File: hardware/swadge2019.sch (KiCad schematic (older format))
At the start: 18 parts, among them SW1 TACTILE, SW2 TACTILE, SW3 TACTILE, SW4 TACTILE, SW5 TACTILE, SW6 TACTILE

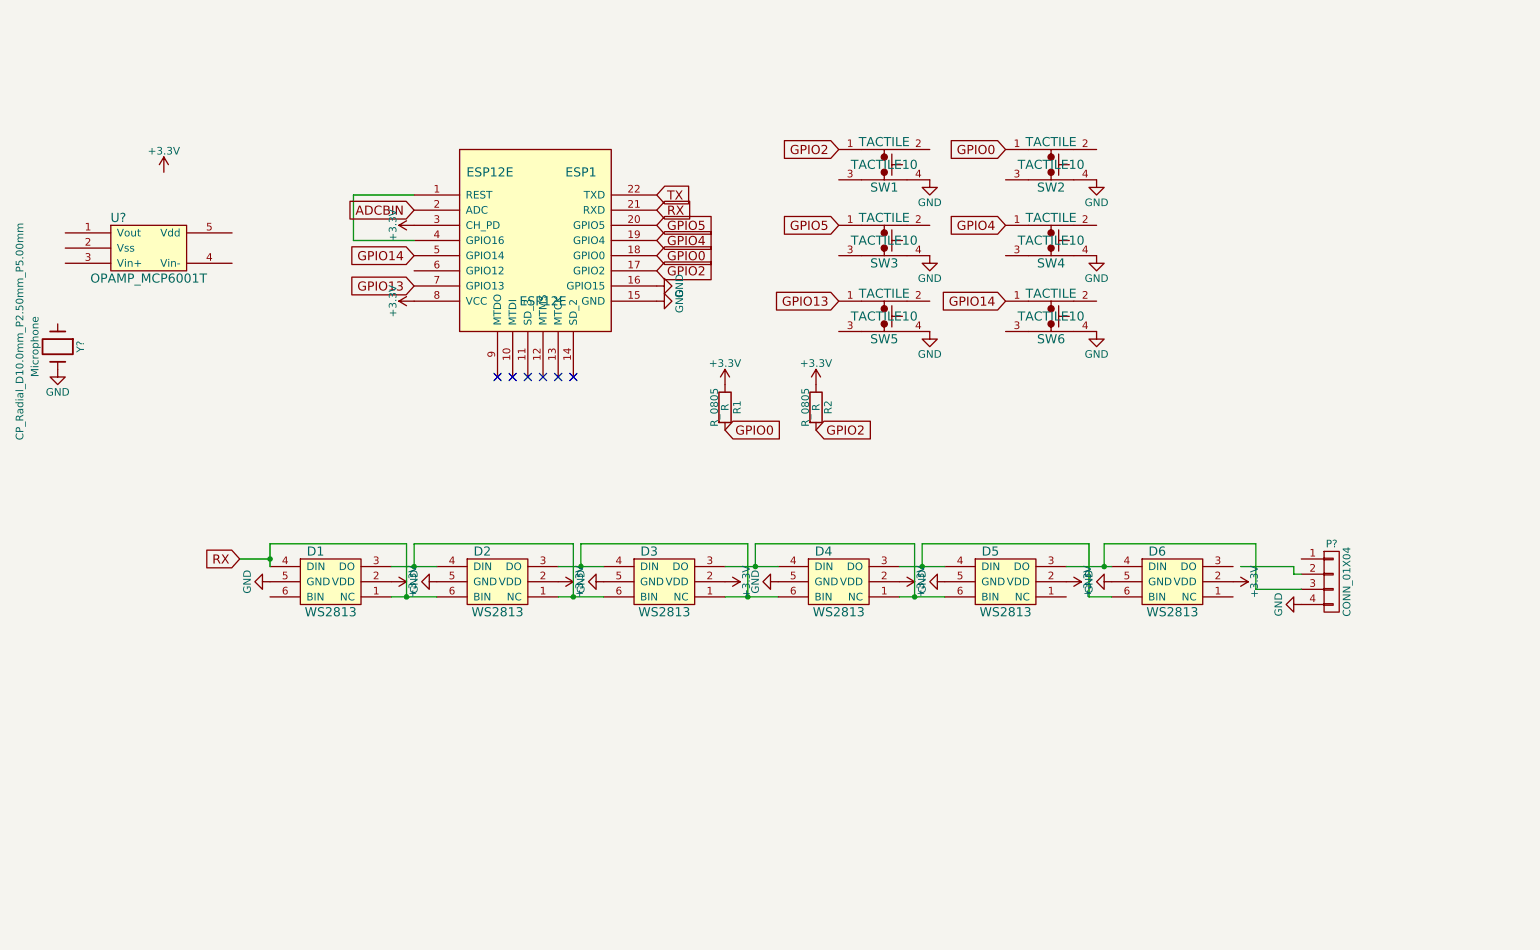
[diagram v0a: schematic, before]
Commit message: bump design
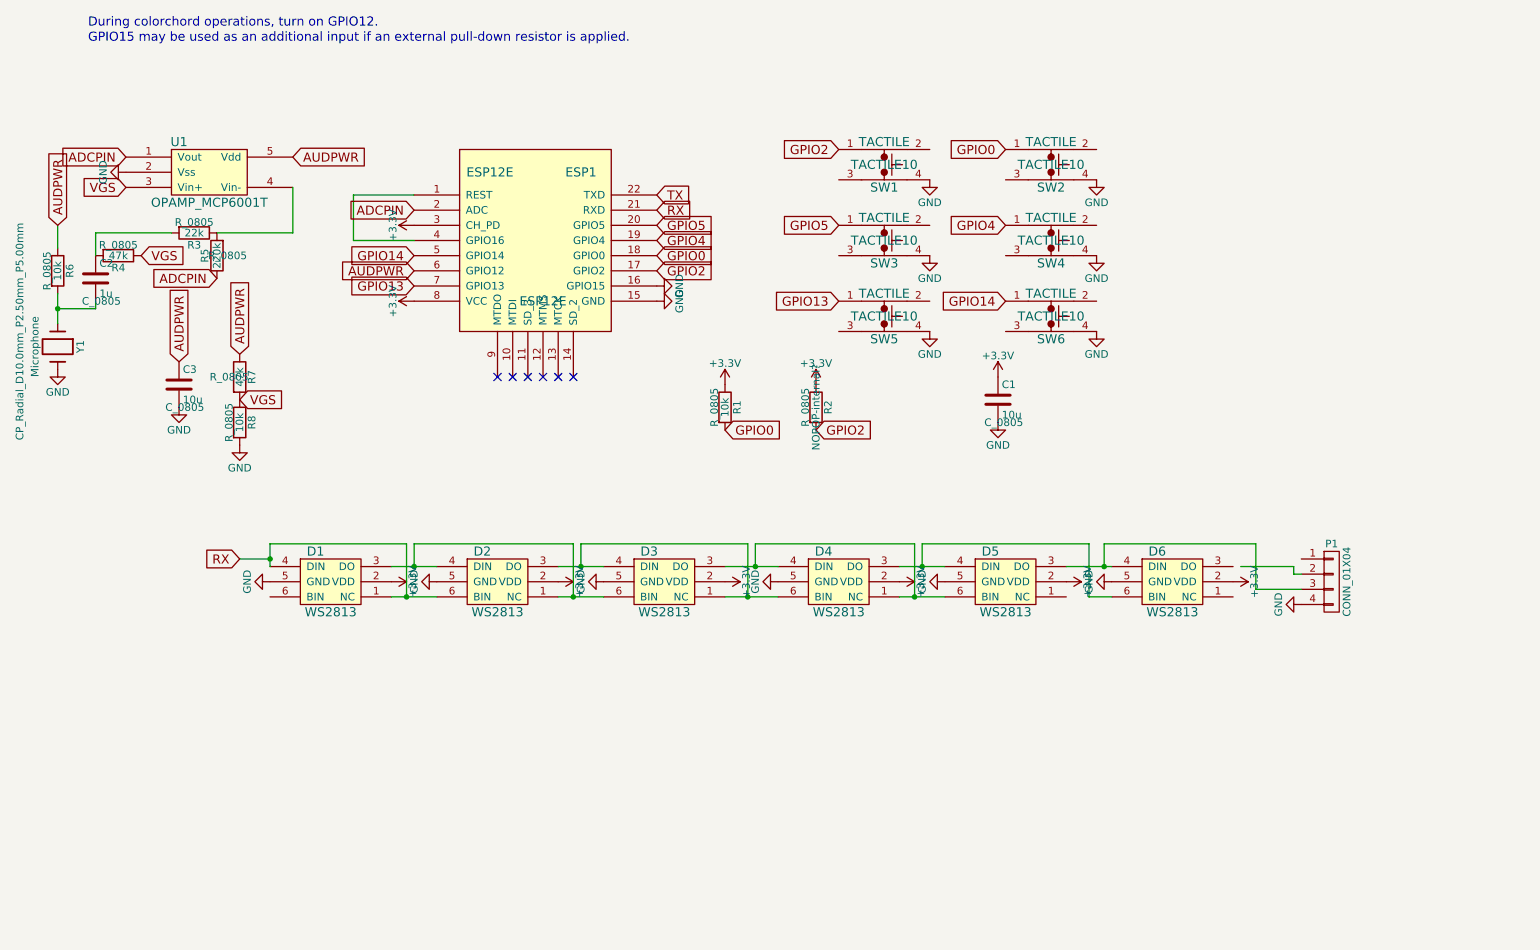
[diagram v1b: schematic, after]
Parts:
- added C1, C3: 10u, C_0805, symbol C
- added C2: 1u, C_0805, symbol C
- added R3: 22k, R_0805, symbol R
- added R4, R7: 47k, R_0805, symbol R
- added R5: 220k, R_0805, symbol R
- added R6, R8: 10k, R_0805, symbol R
- R1: value R -> 10k
- R2: value R -> NOPOP-internal?
- gave numbers to parts that had none: 3
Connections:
- net ADCBIN is gone; now on net ADCPIN: ESP1.2 (ADC)
- net +3V3: now also C1.1
- net GND: now also U1.2 (Vss), C1.2, C3.2, R8.2
- net AUDPWR: now reaches ESP1.6 (GPIO12)
- net AUDPWR: now also U1.5 (Vdd), C3.1, R6.1, R7.1
- net ADCPIN: now reaches U1.1 (Vout)
- net ADCPIN: now also R5.1
- net VGS: now reaches U1.3 (Vin+)
- net VGS: now also R4.1, R7.2, R8.1
- net at U1.4 (Vin-): now also R3.1, R5.2
- net at Y1.1: now also C2.2, R6.2
- new net: C2.1, R3.2, R4.2
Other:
- note added: "During colorchord operations, turn on GPIO12."
- note added: "GPIO15 may be used as an additional input if an external pull-down resistor is applied."
- moved on the sheet: U1

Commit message: update swadge set
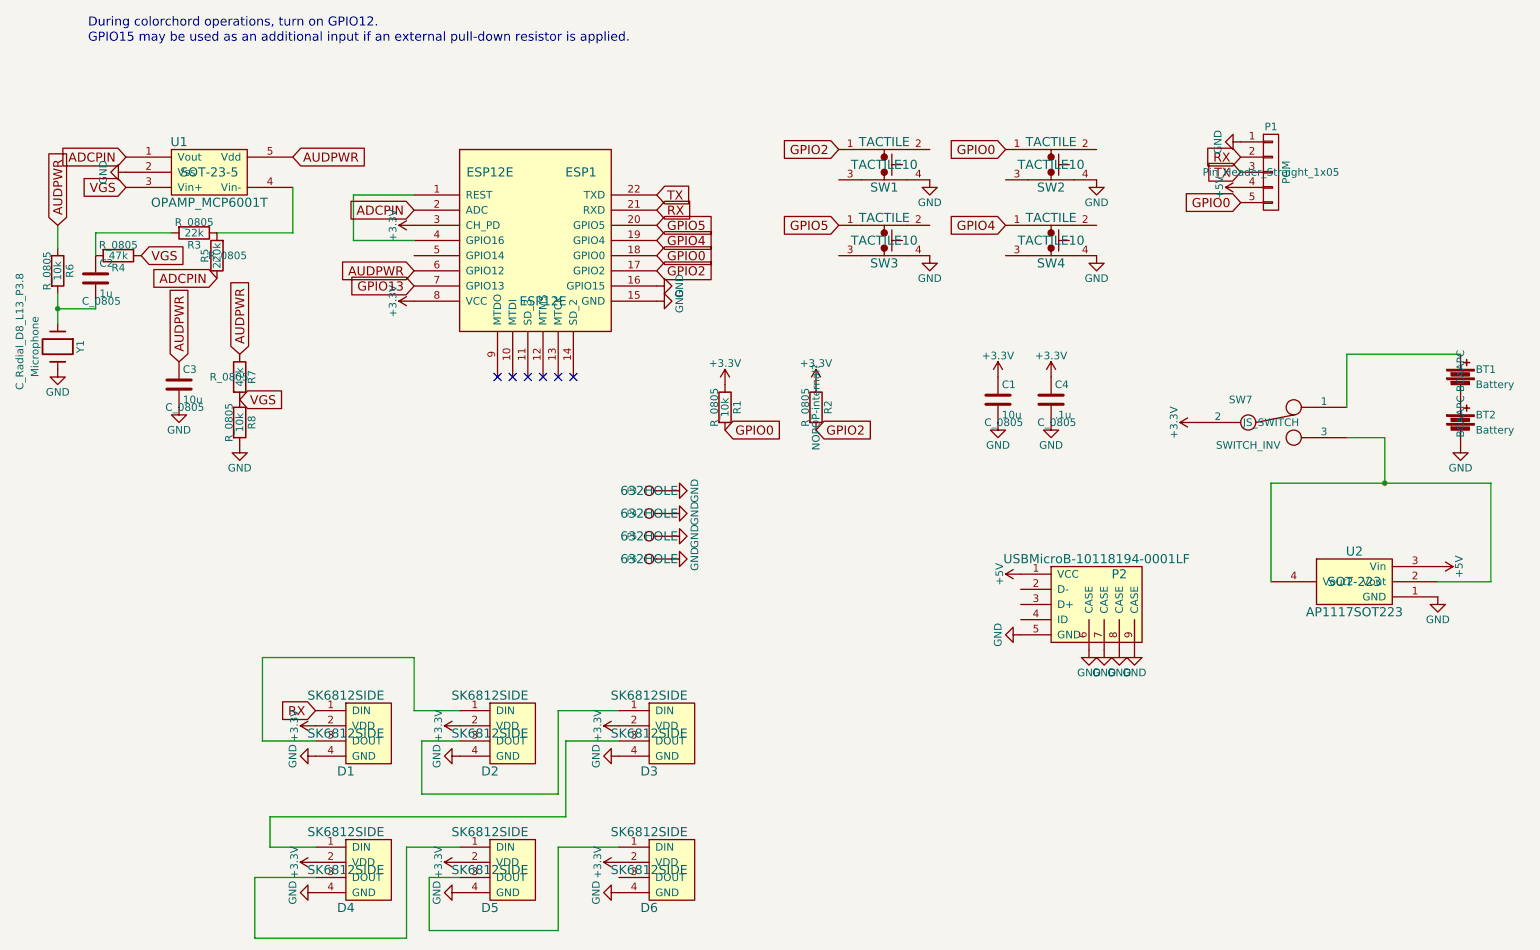
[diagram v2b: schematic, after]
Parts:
- removed D1, D2, D3, D4, D5, D6: WS2813, WS2813, symbol WS2813
- removed P1: CONN_01X04, symbol CONN_01X04
- removed SW5, SW6: TACTILE, TACTILE10, symbol TACTILE
- added BT1, BT2: Battery, BCAAPC, symbol Battery
- added C4: .1u, C_0805, symbol C
- added D1, D2, D3, D4, D5, D6: SK6812SIDE, SK6812SIDE, symbol SK6812SIDE
- added P1: PGM, Pin_Header_Straight_1x05, symbol CONN_01X05
- added P2: USBMicroB-10118194-0001LF, USBMicroB-10118194-0001LF, symbol USBMicroB-10118194-0001LF
- added P3, P4, P5, P6: CONN_1, 632HOLE, symbol CONN_1
- added SW7: SWITCH_INV, JS_SWITCH, symbol SWITCH_INV
- added U2: AP1117SOT223, SOT-223, symbol AP1117SOT223
- U1: footprint (none) -> SOT-23-5
- Y1: footprint CP_Radial_D10.0mm_P2.50mm_P5.00mm -> C_Radial_D8_L13_P3.8
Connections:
- net +3V3: now also C4.1, D1.2 (VDD), D2.2 (VDD), D3.2 (VDD), D4.2 (VDD), D5.2 (VDD), D6.2 (VDD), SW7.2
- net GND: now also BT2.2, C4.2, D1.4 (GND), D2.4 (GND), D3.4 (GND), D4.4 (GND), D5.4 (GND), D6.4 (GND), P1.1 (P1), P2.5 (GND), P2.6 (CASE), P2.7 (CASE), P2.8 (CASE), P2.9 (CASE), P3.1, P4.1, P5.1, P6.1, U2.1 (GND)
- net GPIO0: now also P1.5 (P5)
- net RX: now also D1.1 (DIN), P1.2 (P2)
- net TX: now also P1.3 (P3)
- net GPIO14: no longer names the net of ESP1.5 (GPIO14)
- new net: D1.3 (DOUT), D2.1 (DIN)
- new net: D2.3 (DOUT), D3.1 (DIN)
- new net: D3.3 (DOUT), D4.1 (DIN)
- new net: D4.3 (DOUT), D5.1 (DIN)
- new net: D5.3 (DOUT), D6.1 (DIN)
- new net: BT1.1, SW7.1
- new net: SW7.3, U2.2 (Vout), U2.4 (Vout2)
- new net: BT1.2, BT2.1
- new net +5V: P1.4 (P4), P2.1 (VCC), U2.3 (Vin)
